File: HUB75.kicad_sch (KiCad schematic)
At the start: 12 parts, among them J2 Conn_02x08_Odd_Even, U10 SN74LVC8T245, U11 SN74LVC8T245, U2 ICE40HX8K-BG121

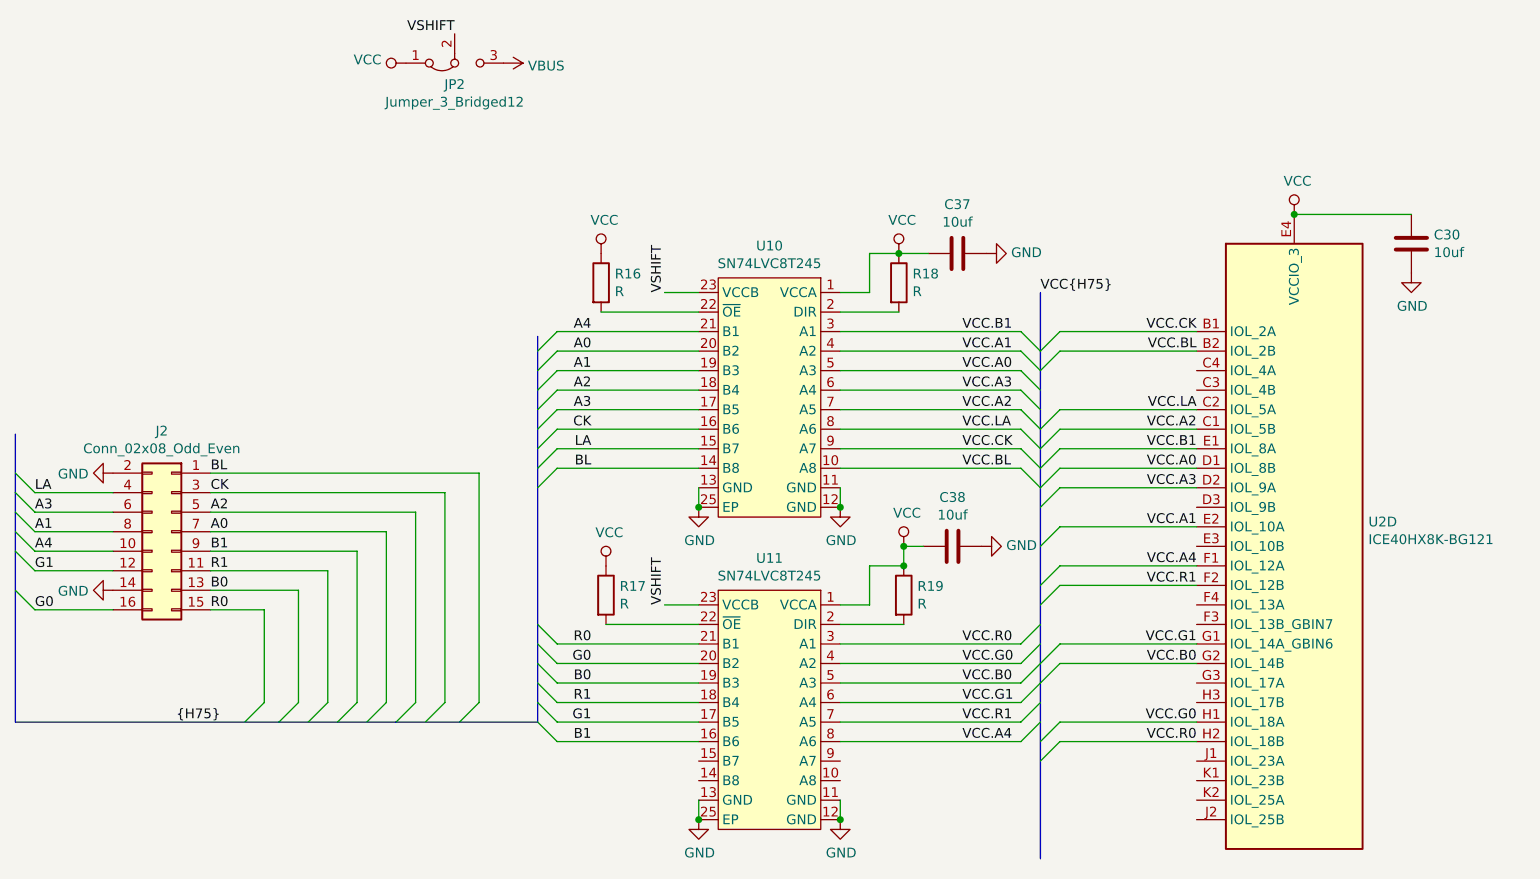
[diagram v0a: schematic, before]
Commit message: Routing changes, pullups, etc
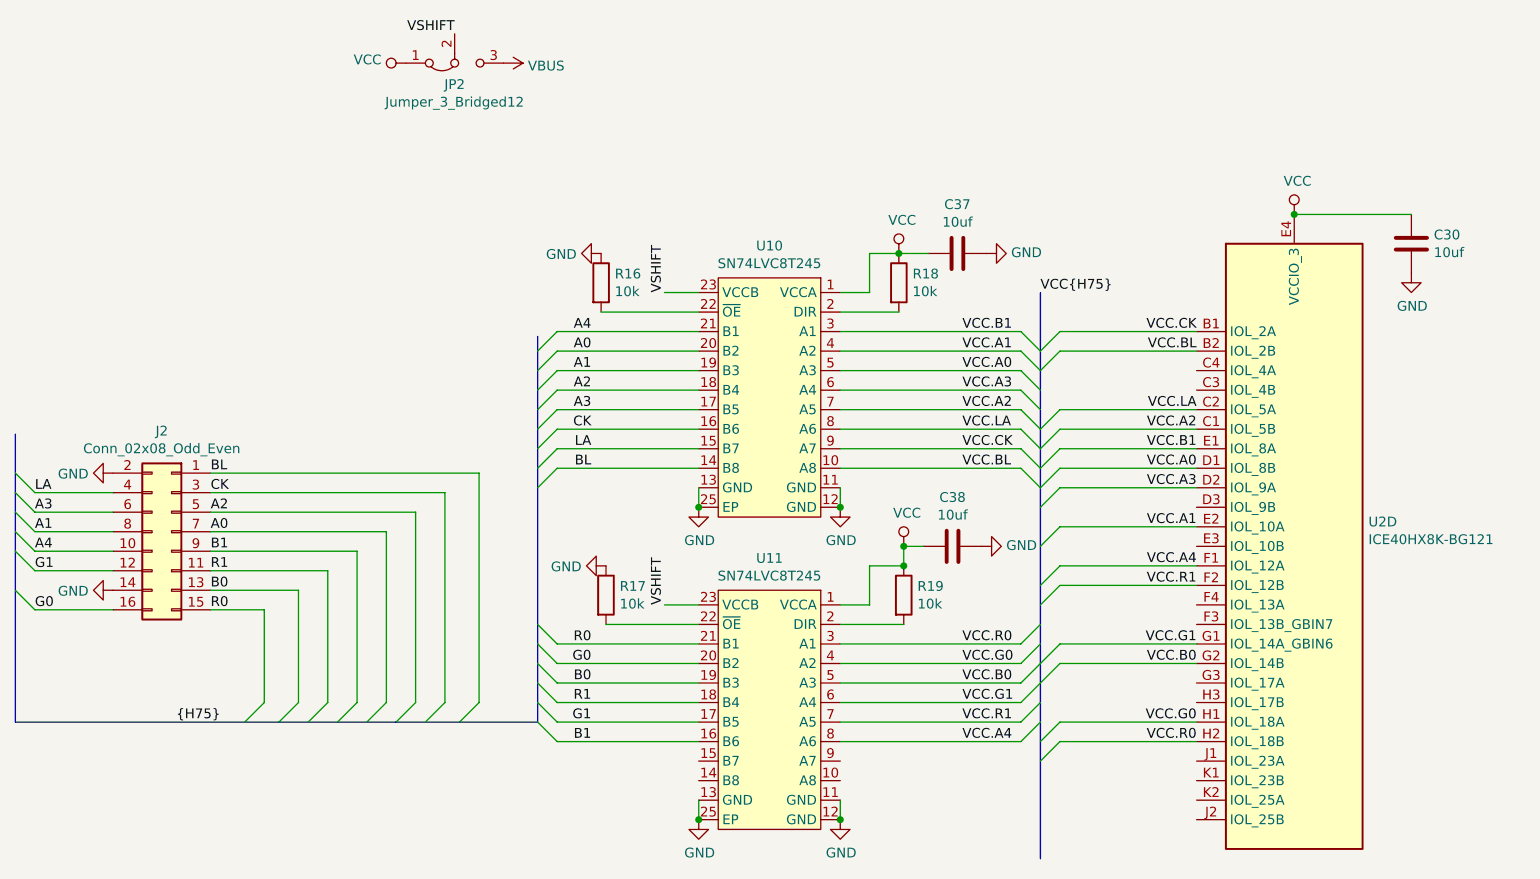
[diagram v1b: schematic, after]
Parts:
- C30, C37, C38, J2, JP2, U10, U11, U2: Source (none) -> ANY
- R16, R17, R18, R19: value R -> 10k; Source (none) -> ANY
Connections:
- net GND: now also R16.1, R17.1
- net VCC: no longer R16.1, R17.1
